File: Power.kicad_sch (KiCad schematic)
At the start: 14 parts, among them J1 USB_B_Micro, J2 Conn_01x02, U1 XC6206PxxxMR, U7 TPS61040DBV

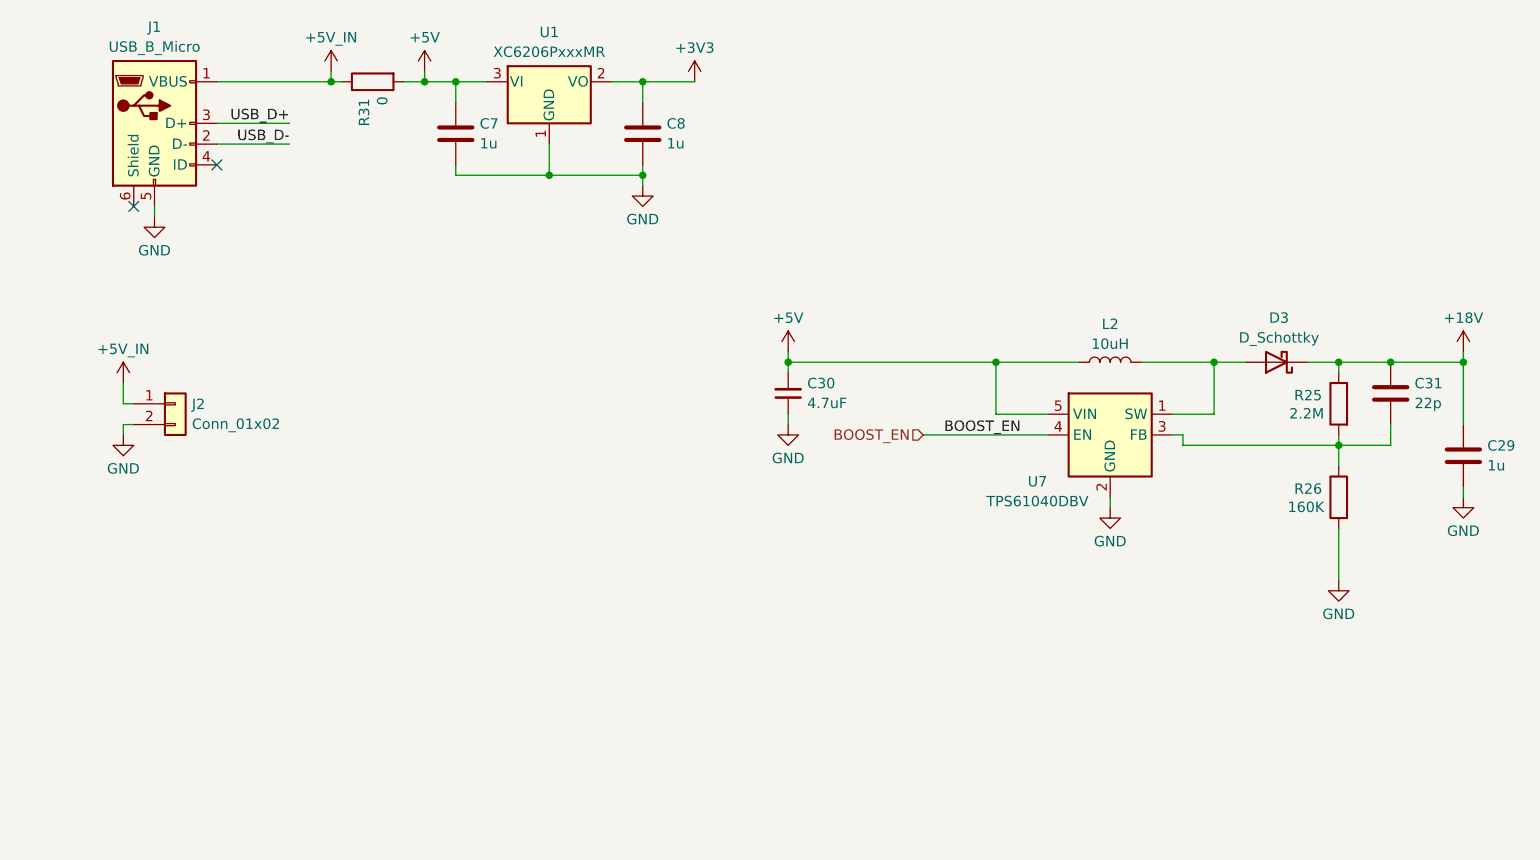
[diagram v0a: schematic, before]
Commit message: Routing
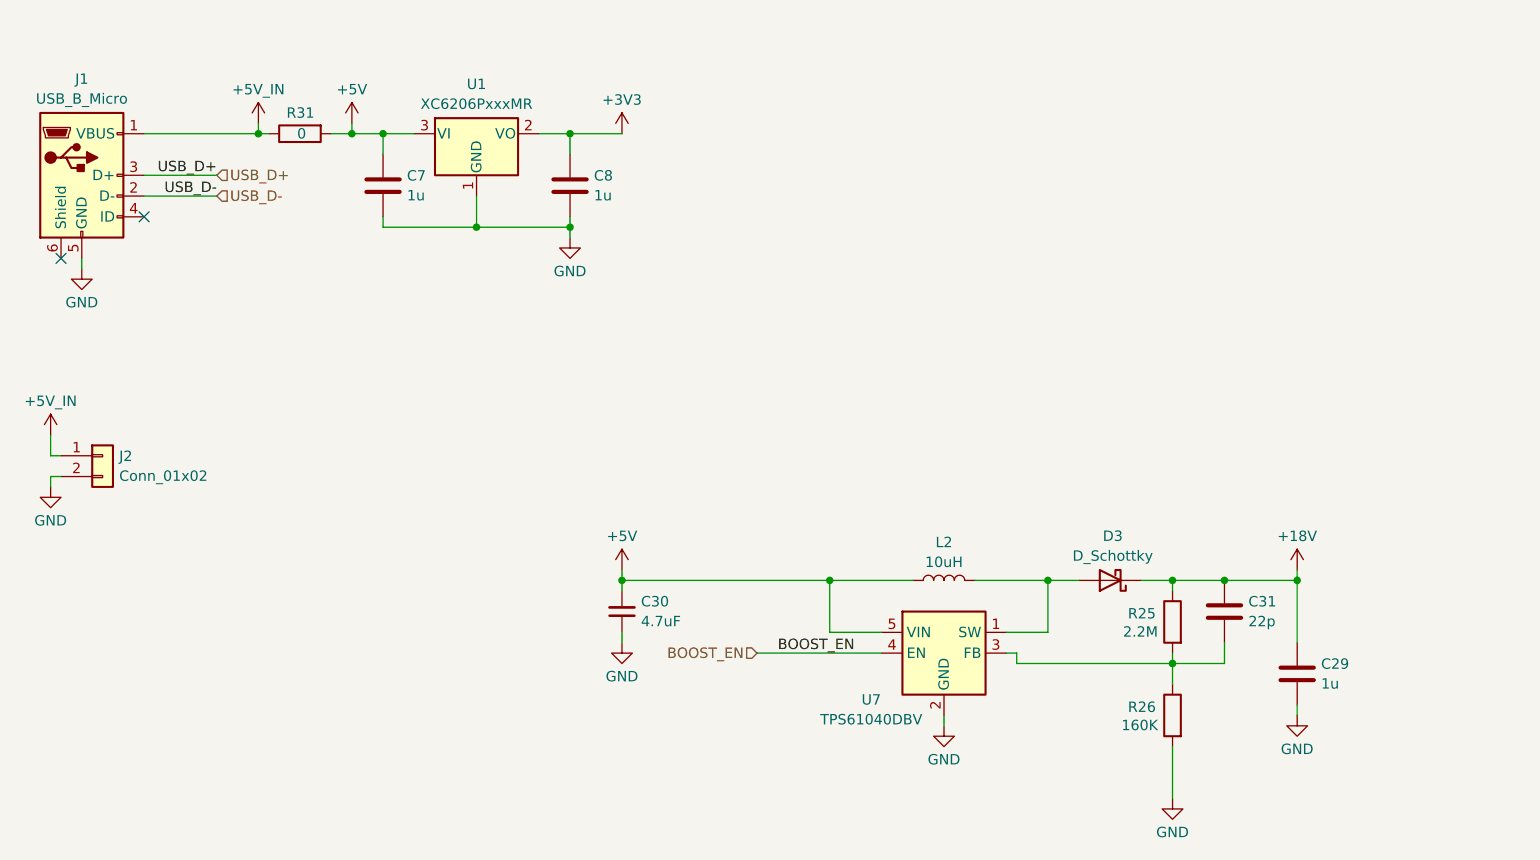
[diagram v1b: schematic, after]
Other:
- moved on the sheet: C29, C30, C31, C7, C8, D3, J1, J2, L2, R25, R26, R31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
